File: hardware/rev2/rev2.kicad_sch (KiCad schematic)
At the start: 2 parts, among them J1 Conn_Coaxial_Small

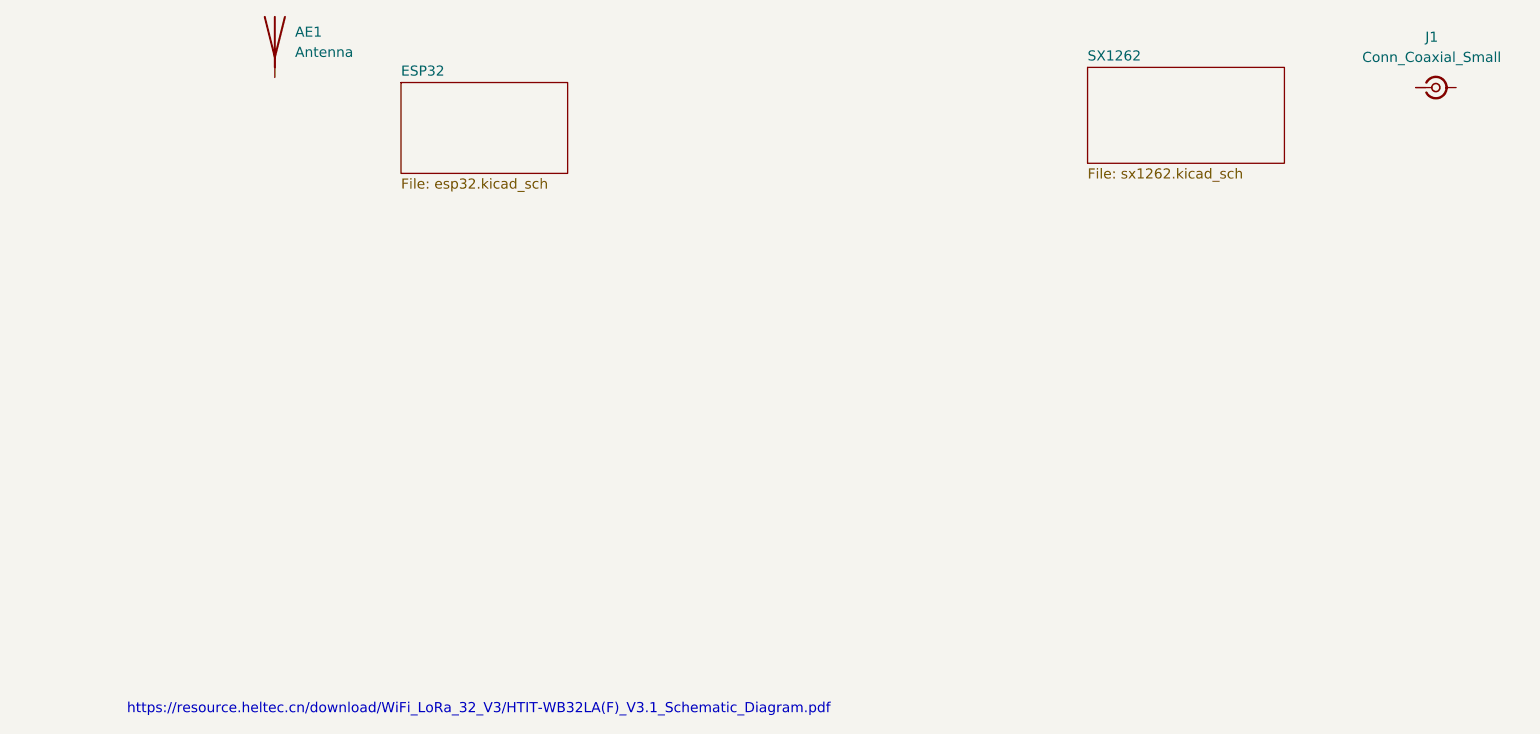
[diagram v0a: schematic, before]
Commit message: did some schematic stuff
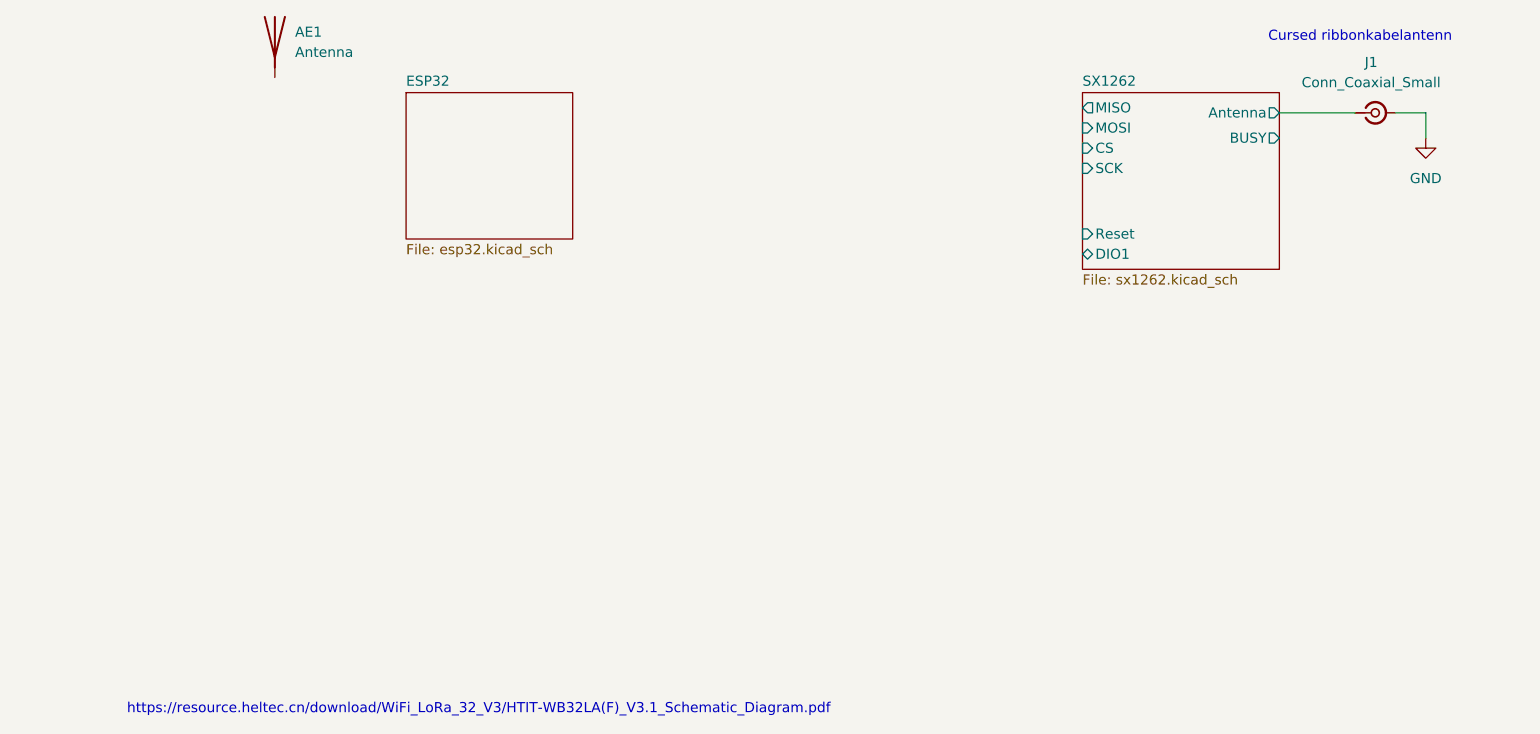
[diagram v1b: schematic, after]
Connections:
- net SX1262/Antenna: now reaches J1.1 (In)
- net GND: now reaches J1.2 (Ext)
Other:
- sheet SX1262 ports: added Antenna, BUSY, CS, DIO1, MISO, MOSI, Reset, SCK; removed none
- note added: "Cursed ribbonkabelantenn"
- moved on the sheet: J1
